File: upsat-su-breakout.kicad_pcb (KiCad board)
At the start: 2 copper layers, 36 x 26 mm, 9 parts, among them P1 SU, P2 EPS, P3 OBC, P4 RBF, P5 STM_0, P6 STM_1, P7 STM_2, P8 STM_3, P9 STM_4

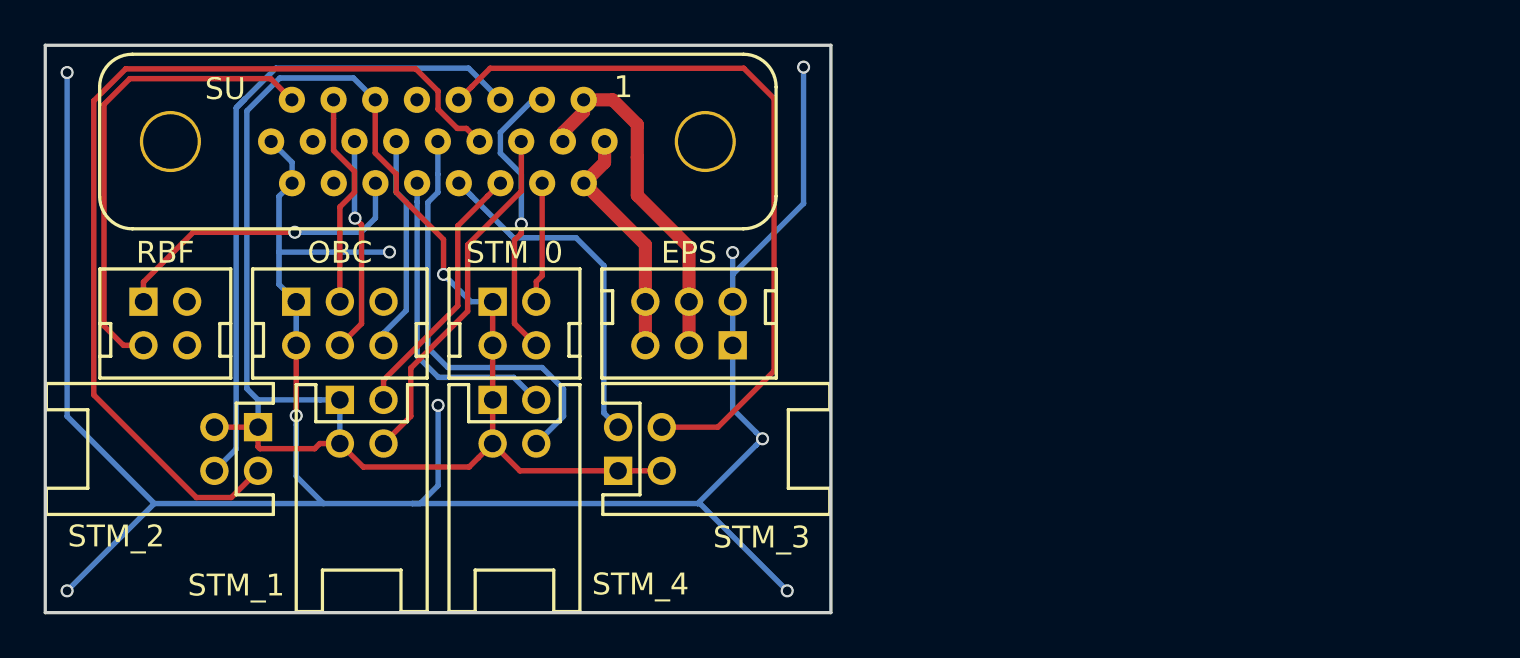
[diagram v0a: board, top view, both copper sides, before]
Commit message: Update layout for better fitting.
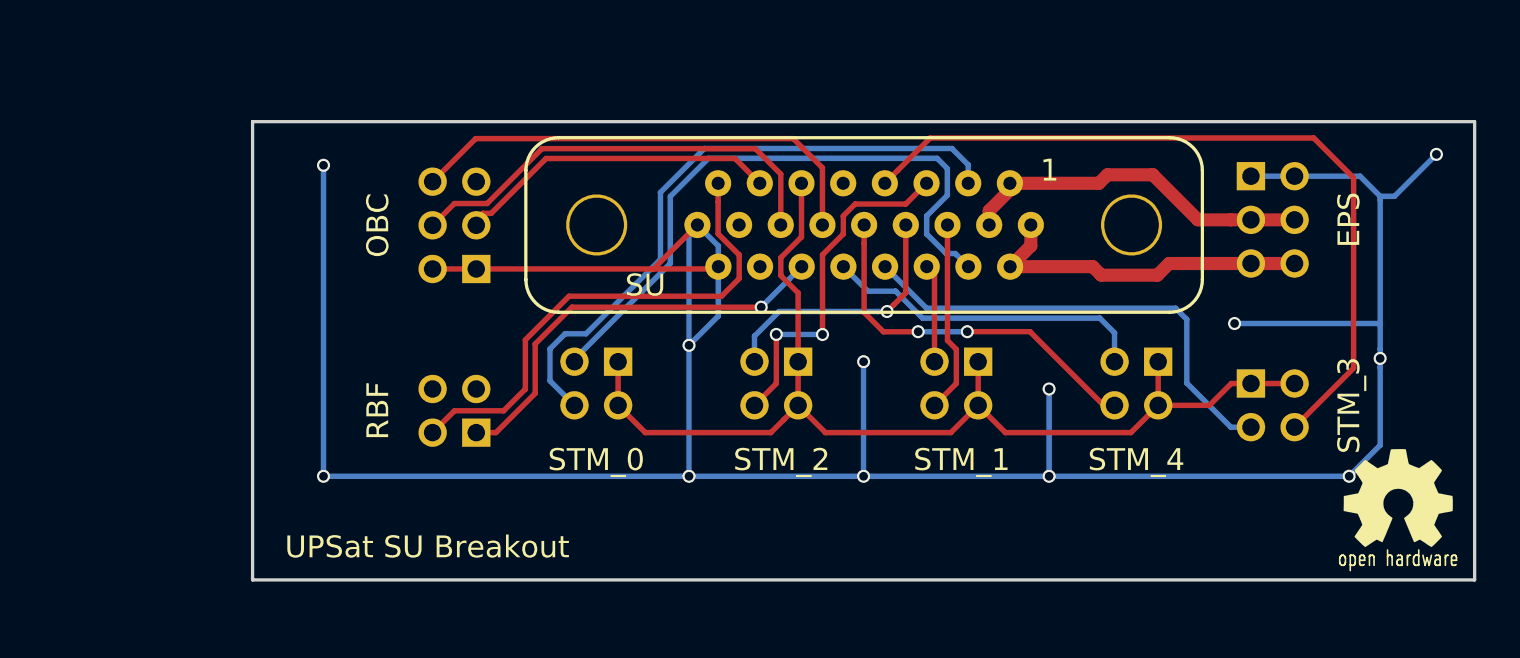
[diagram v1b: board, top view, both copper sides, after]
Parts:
- added G***: LOGO, w_logo:Logo_silk_OSHW_6x6mm, F.Cu at (195.2, 110.5)
- P2, P3: footprint hrs-df11:hrs-df11-6dp-2dsa -> hrs-df11:hrs-df11-6dp-2ds; moved to B.Cu
- P4, P5: footprint hrs-df11:hrs-df11-4dp-2dsa -> hrs-df11:hrs-df11-4dp-2ds; moved to B.Cu
- P6, P7, P8, P9: moved to B.Cu
- moved P8 29.1 mm to (189.5, 106.2), turned to 90 degrees
- moved P9 28.6 mm to (183.2, 105.2), turned to 0 degrees
- moved P6 27.3 mm to (175.0, 105.2), turned to 0 degrees
- moved P2 27.2 mm to (189.5, 97.8), turned to 90 degrees
- moved P7 24.9 mm to (166.8, 105.2), turned to 0 degrees
- moved P1 19.9 mm to (170.8, 98.0)
- moved P4 13.8 mm to (152.0, 106.5), turned to 270 degrees
- moved P3 6.91 mm to (152.0, 98.0), turned to 270 degrees
- moved P5 4.65 mm to (158.5, 105.2), turned to 0 degrees
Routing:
- net (no net): track 0.00 -> 55.0 mm
- net /STM_TH_RET_2: track 43.6 -> 12.0 mm, vias 0 -> 1
- net /GND: track 110.2 -> 134.4 mm, vias 9 -> 12
- net /STM_TH_RET_0: track 5.54 -> 28.9 mm
- net /STM_SHIELD: track 68.9 -> 51.4 mm, vias 1 -> 0
- net /STM_TH_GO_0: track 13.2 -> 29.0 mm, vias 1 -> 0
- net /STM_TH_GO_2: track 31.0 -> 16.0 mm, vias 0 -> 2
- net /MNLP_TH_RET: track 9.96 -> 21.9 mm
- net /MNLP_RX: track 9.89 -> 20.2 mm, vias 1 -> 0
- net /STM_TH_RET_1: track 12.2 -> 4.50 mm
- net /STM_TH_GO_1: track 16.5 -> 8.85 mm
- net /BIAS_DISARM_GND: track 14.3 -> 19.4 mm
- net /MNLP_TX: track 9.93 -> 14.9 mm
- net /+5: track 10.9 -> 15.7 mm
- net /STM_TH_RET_3: track 16.7 -> 21.5 mm
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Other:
- board size 36 x 26 mm -> 56 x 21 mm
- board text added: "UPSat SU Breakout"
